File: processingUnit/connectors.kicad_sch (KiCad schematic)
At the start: 10 parts, among them J101 Conn_01x05, J102 Conn_01x04, J301 Conn_01x10, J309 Conn_01x02

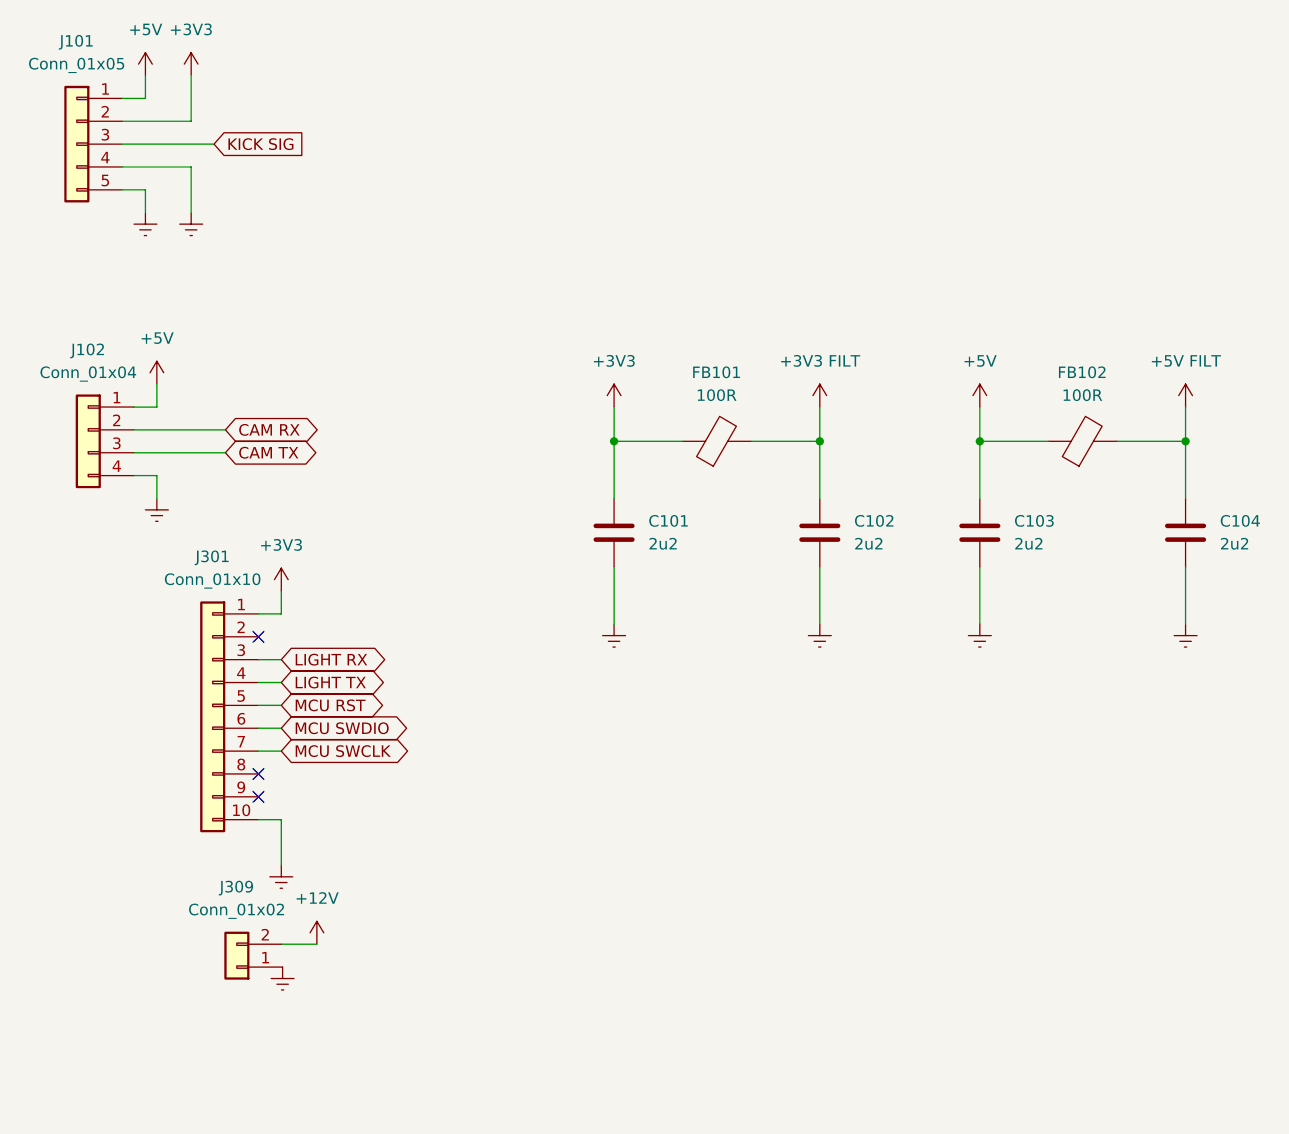
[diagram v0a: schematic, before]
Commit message: L3
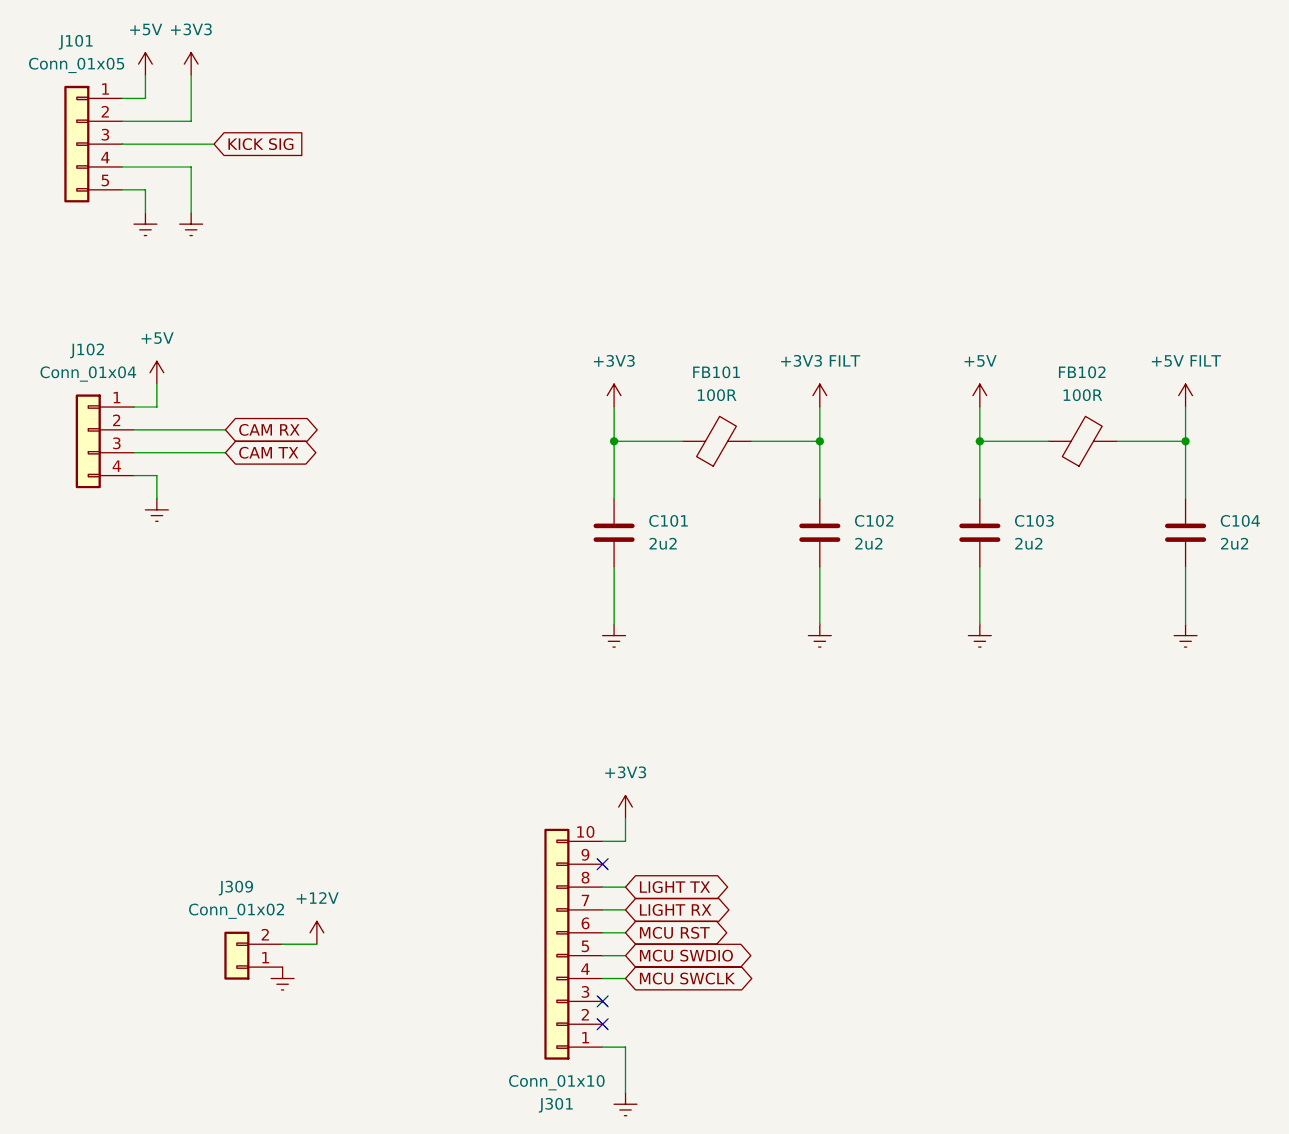
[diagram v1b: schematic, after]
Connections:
- net +3V3: now also J301.10 (Pin_10); no longer J301.1 (Pin_1)
- net GNDREF: now also J301.1 (Pin_1); no longer J301.10 (Pin_10)
- net LIGHT RX: now also J301.7 (Pin_7); no longer J301.3 (Pin_3)
- net LIGHT TX: now also J301.8 (Pin_8); no longer J301.4 (Pin_4)
- net MCU RST: now also J301.6 (Pin_6); no longer J301.5 (Pin_5)
- net MCU SWCLK: now also J301.4 (Pin_4); no longer J301.7 (Pin_7)
- net MCU SWDIO: now also J301.5 (Pin_5); no longer J301.6 (Pin_6)
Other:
- moved on the sheet: J301
